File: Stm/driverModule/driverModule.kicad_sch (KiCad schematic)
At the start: 6 parts, among them U101 STM32G431KBTx, U102 ADM7171ACPZ-3.0-R7, U103 TJA1051T-3

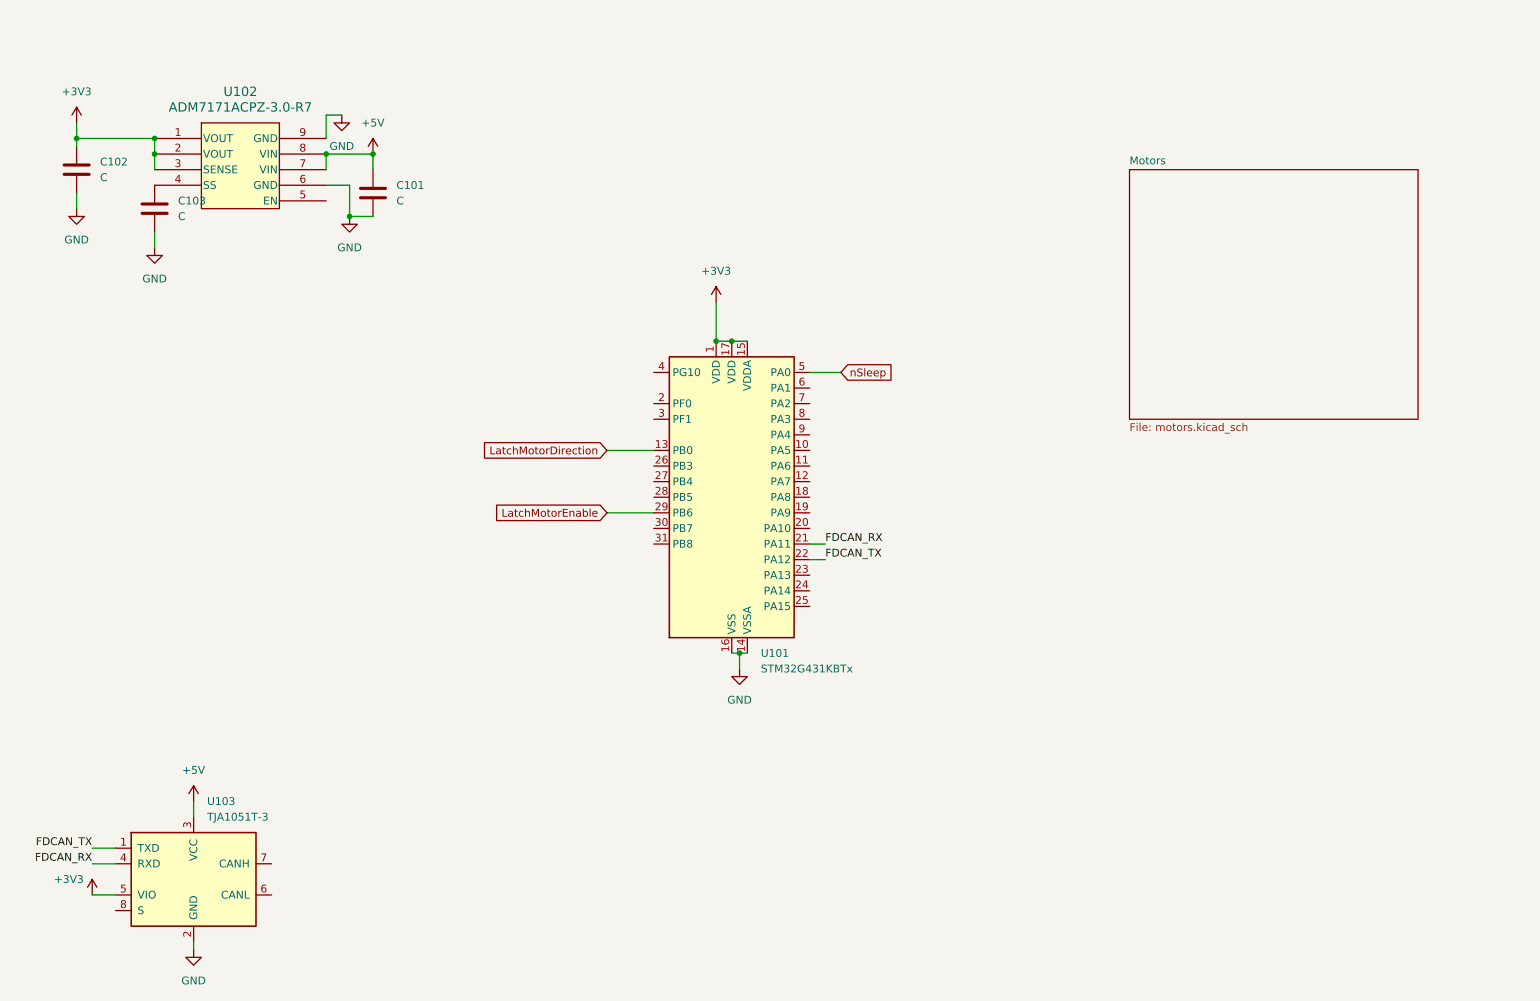
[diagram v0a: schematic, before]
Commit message: Add Headers
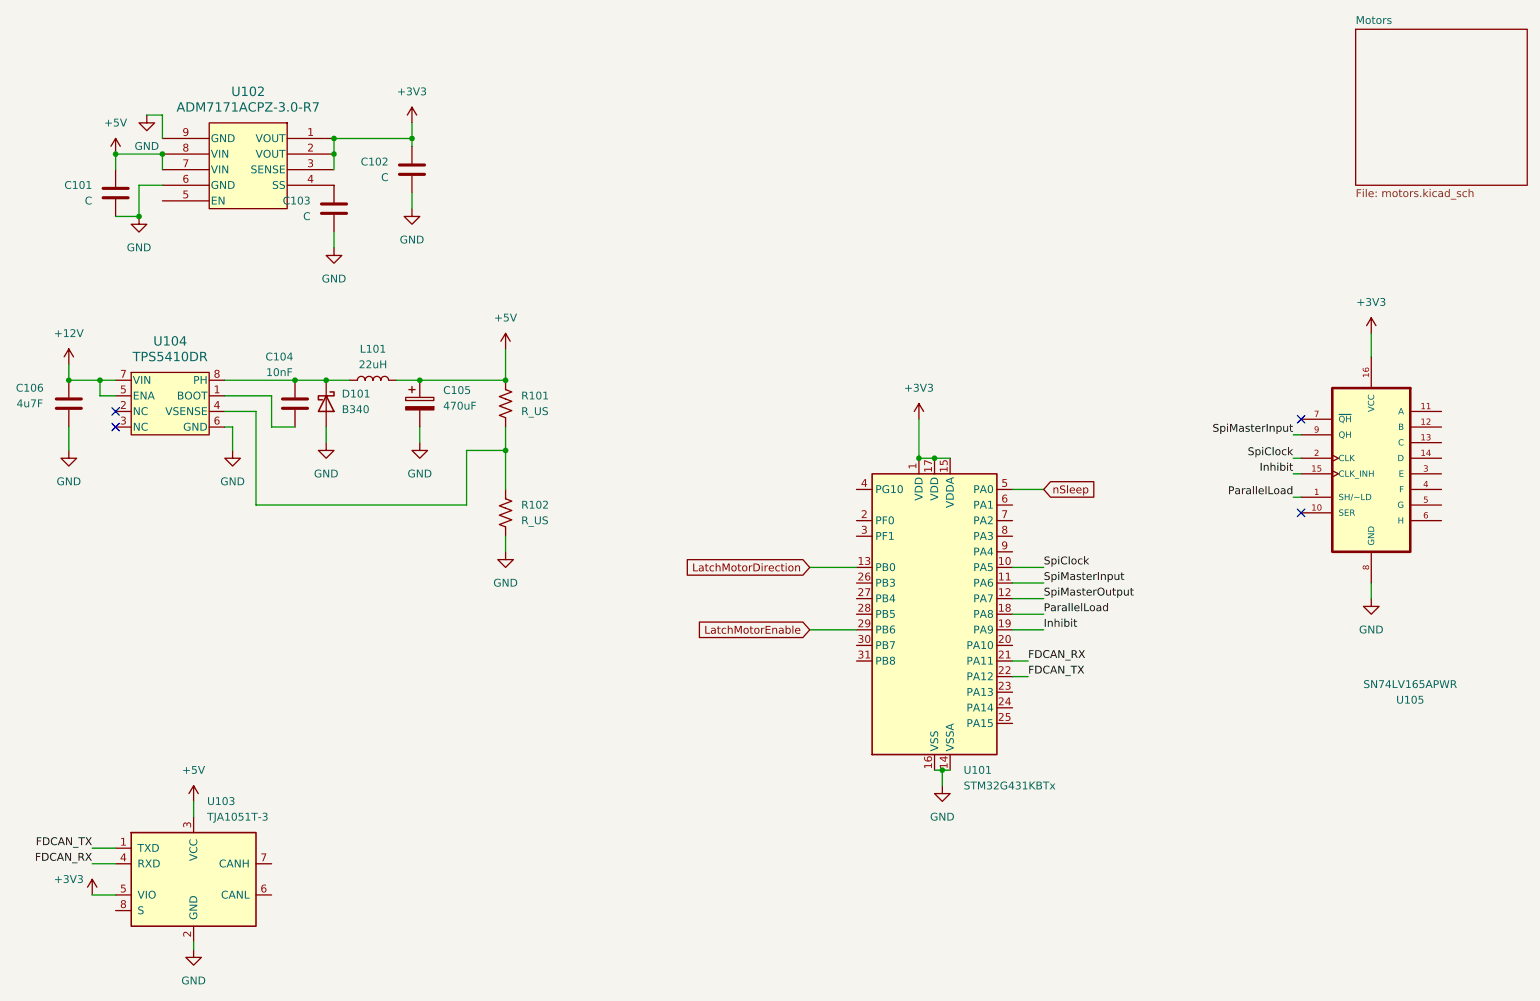
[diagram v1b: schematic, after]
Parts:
- added C104: 10nF, symbol Device:C
- added C105: 470uF, symbol Device:C_Polarized
- added C106: 4u7F, symbol Device:C
- added D101: B340, Diode_SMD:D_SMC, symbol Diode:B340
- added L101: 22uH, symbol Device:L
- added R101, R102: R_US, symbol Device:R_US
- added U104: TPS5410DR, Package_SO:SOIC-8-N7_3.9x4.9mm_P1.27mm, symbol Local_symbols:TPS5410DR
- added U105: SN74LV165APWR, Package_SO:TSSOP-16_4.4x5mm_P0.65mm, symbol Local_symbols:SN74LV165APWR
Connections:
- net +3V3: now also U105.16 (VCC)
- net +5V: now also C105.1, L101.2, R101.1
- net GND: now also C105.2, C106.1, D101.2 (A), R102.2, U104.6 (GND), U105.8 (GND)
- net SpiClock: now reaches U101.10 (PA5)
- net SpiClock: now also U105.2 (CLK)
- net SpiMasterInput: now reaches U101.11 (PA6)
- net SpiMasterInput: now also U105.9 (QH)
- net SpiMasterOutput: now reaches U101.12 (PA7)
- net ParallelLoad: now reaches U101.18 (PA8)
- net ParallelLoad: now also U105.1 (SH/~LD)
- net Inhibit: now reaches U101.19 (PA9)
- net Inhibit: now also U105.15 (CLK_INH)
- new net: C104.1, U104.1 (BOOT)
- new net: R101.2, R102.1, U104.4 (VSENSE)
- new net: C104.2, D101.1 (K), L101.1, U104.8 (PH)
- new net +12V: C106.2, U104.5 (ENA), U104.7 (VIN)
- no-connect marks 0 -> 4
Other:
- moved on the sheet: C101, C102, C103, U101, U102
